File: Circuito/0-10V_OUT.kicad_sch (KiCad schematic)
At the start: 6 parts, among them U4 AT3H4B-CUH-S

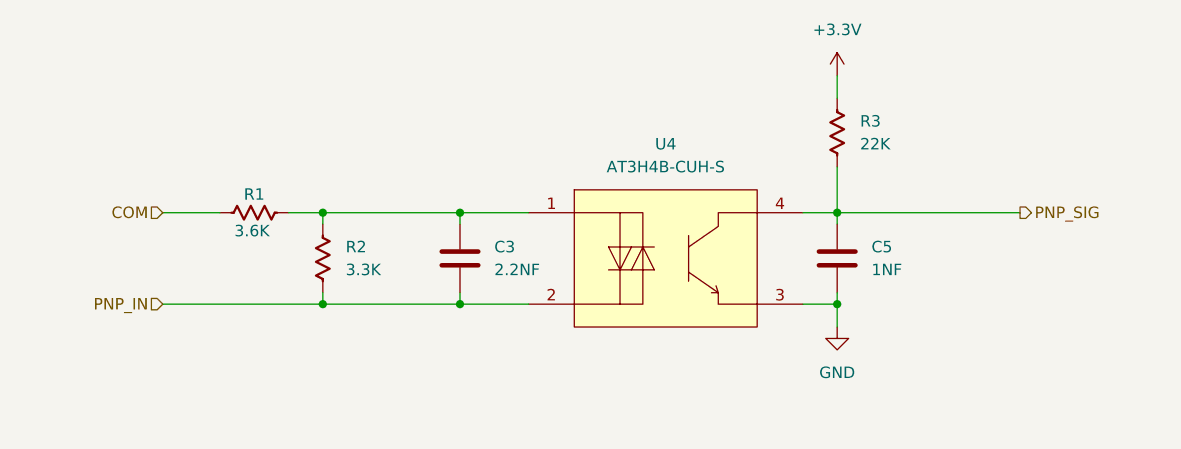
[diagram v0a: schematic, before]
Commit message: commit
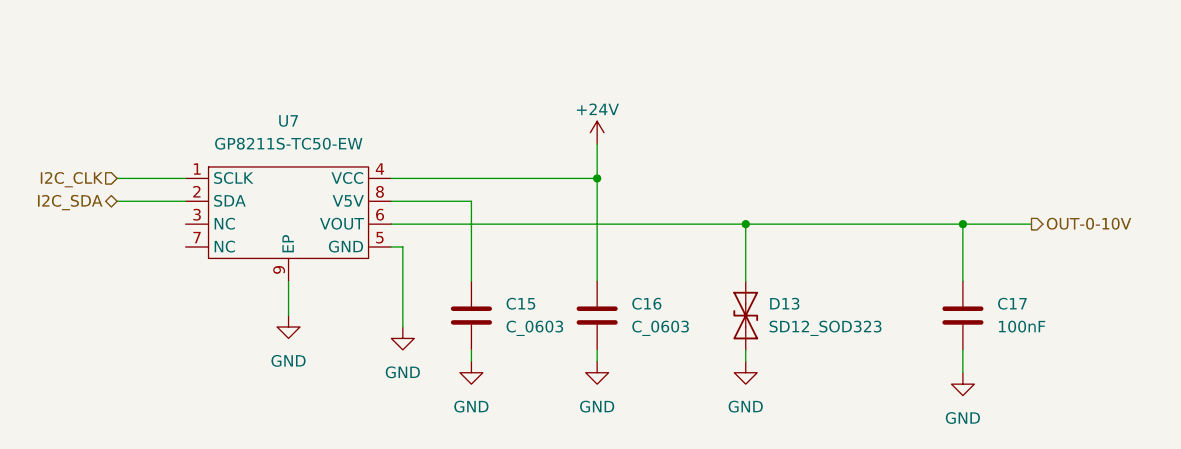
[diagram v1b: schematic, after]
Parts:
- removed C3: 2.2NF, PCM_Capacitor_SMD_AKL:C_0603_1608Metric, symbol Capacitor_AKL:C_0603
- removed C5: 1NF, PCM_Capacitor_SMD_AKL:C_0603_1608Metric, symbol Capacitor_AKL:C_0603
- removed R1: 3.6K, PCM_Resistor_SMD_AKL:R_0603_1608Metric, symbol Resistor_US_AKL:R_0603
- removed R2: 3.3K, PCM_Resistor_SMD_AKL:R_0603_1608Metric, symbol Resistor_US_AKL:R_0603
- removed R3: 22K, PCM_Resistor_SMD_AKL:R_0603_1608Metric, symbol Resistor_US_AKL:R_0603
- removed U4: AT3H4B-CUH-S, easyeda2kicad:SSOP-4_L2.7-W4.6-P1.27-LS7.0-TL, symbol easyeda2kicad:AT3H4B-CUH-S
- added C15, C16: C_0603, PCM_Capacitor_SMD_AKL:C_0603_1608Metric, symbol Capacitor_AKL:C_0603
- added C17: 100nF, PCM_Capacitor_SMD_AKL:C_0603_1608Metric, symbol Capacitor_AKL:C_0603
- added D13: SD12_SOD323, Diode_SMD:D_SOD-323, symbol Diode:SD12_SOD323
- added U7: GP8211S-TC50-EW, EasyEDA:ESOP-8_L4.9-W3.9-P1.27-LS6.0-BL-EP, symbol EasyEDA:GP8211S-TC50-EW
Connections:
- net GND: now also C15.2, C16.2, C17.2, D13.1 (A1), U7.5 (GND), U7.9 (EP)
- new net: C15.1, U7.8 (V5V)
- new net +24V: C16.1, U7.4 (VCC)
- new net I2C_CLK: U7.1 (SCLK)
- new net I2C_SDA: U7.2 (SDA)
- new net OUT-0-10V: C17.1, D13.2 (A2), U7.6 (VOUT)
